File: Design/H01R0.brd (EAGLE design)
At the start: 34.6 x 30 mm, 27 parts, among them P1 HEXABIT_17.32, Q1 MMBT3904LT1, Q2 MMBT3904LT1, Q3 MMBT3904LT1, U1 STM32G0B1CEU6NUFQFPN48_STM32_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, X1 XTALL_CSTCE8M00G52

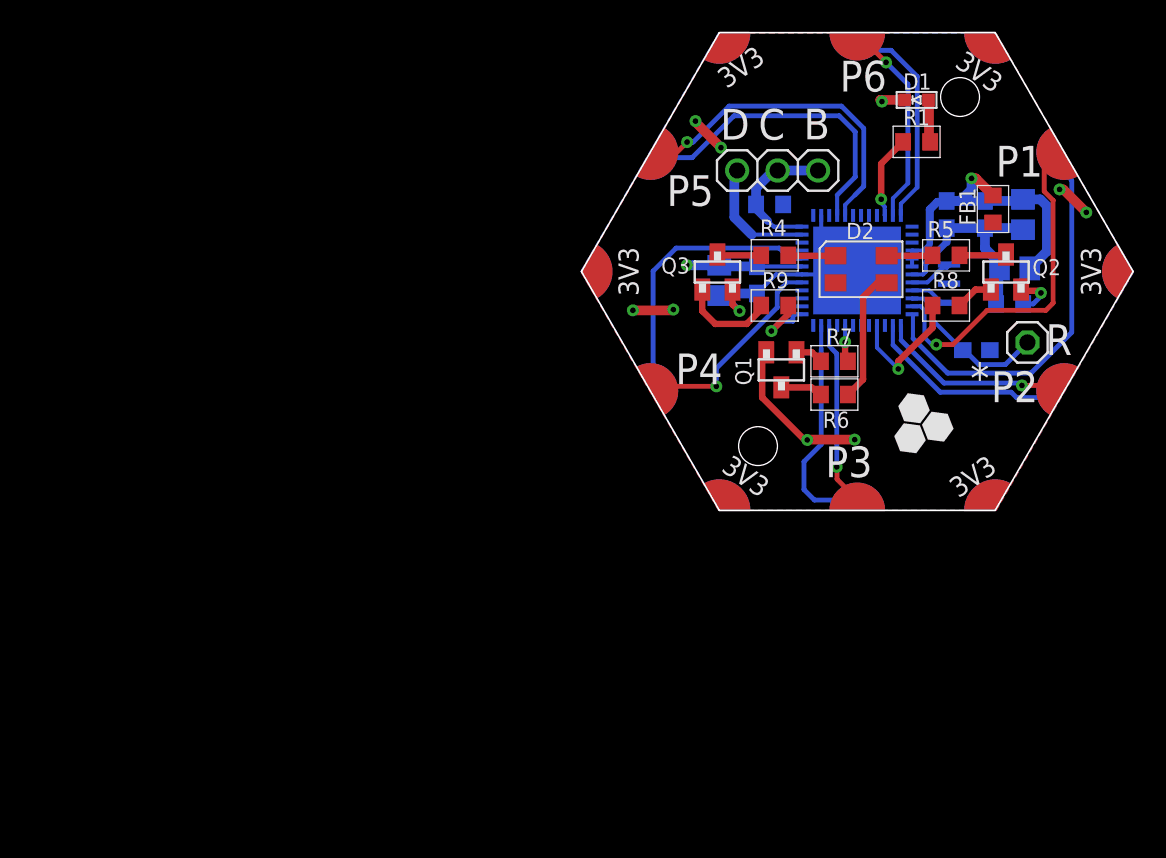
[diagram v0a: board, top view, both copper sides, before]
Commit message: -Improving the Layout Design
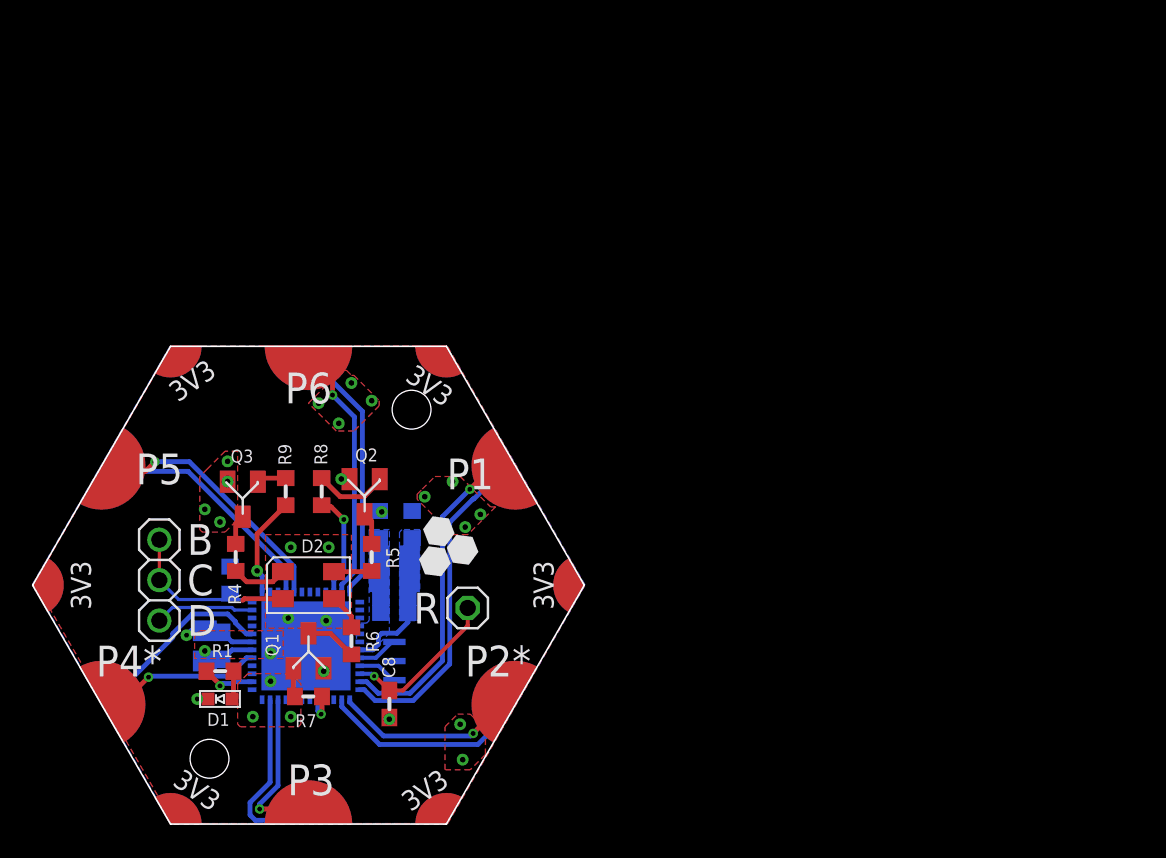
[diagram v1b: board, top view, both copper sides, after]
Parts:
- D1: value VLMS1300-GS08 -> RED
- FB1: device HEXABITZ_RCLS:FB-TDK_MMZ1608Y300B -> HEXABITZ_RCLS:FB-0603
- U1: value STM32G0B1CEU6NUFQFPN48_STM32_STM -> STM32G0B1CEU6N; device HEXABITZ_ICs:UFQFPN48_STM32_STM -> HEXABITZ_ICs:HEXABITZ_ICS_QFN_B1CEU6_STM-L
- moved D1 57.7 mm to (-5.56, 7.78)
- moved R1 54.9 mm to (-5.56, 9.53)
- moved JP2 46.6 mm to (-9.37, 15.2), turned to 270 degrees
- moved C2 45.7 mm to (5.40, 15.2), turned to 180 degrees
- moved C6 44.2 mm to (5.40, 14.1), turned to 180 degrees
- moved FB1 43.3 mm to (4.45, 18.7), flipped to the bottom, turned to 90 degrees
- moved C8 43.0 mm to (5.08, 7.46), flipped to the top, turned to 270 degrees
- moved C7 43.0 mm to (5.40, 16.7), turned to 180 degrees
- moved C5 42.8 mm to (5.40, 13.2), turned to 180 degrees
- moved Q2 42.7 mm to (3.53, 20.5), turned to 180 degrees
- moved X1 42.1 mm to (5.40, 10.2)
- moved U1 41.9 mm to (-0.16, 11.1)
- moved R3 41.3 mm to (-4.92, 15.2), turned to 270 degrees
- moved R8 40.9 mm to (0.83, 20.8), turned to 90 degrees
- moved R5 40.8 mm to (3.97, 16.7), turned to 90 degrees
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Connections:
- net BLED: now also U1.17; no longer U1.20
- net GLED: now also U1.46; no longer U1.16
- net GND: no longer U1.1, U1.2, U1.37, U1.38
- net N$7: now also U1.26; no longer U1.46
- net RLED: now also U1.37; no longer U1.25
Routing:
- net GND: track 33.1 -> 4.73 mm, vias 11 -> 27
- net VDDA: track 21.0 -> 0.00 mm, vias 1 -> 0
- net VSSA: track 14.3 -> 4.60 mm
- net USART4_RX: track 29.7 -> 20.6 mm
- net N$8: track 8.36 -> 2.25 mm
- net USART1_RX: track 17.7 -> 11.8 mm
- net USART3_RX: track 17.1 -> 11.8 mm
- net USART5_TX: track 21.4 -> 16.1 mm
- net USART5_RX: track 19.5 -> 15.0 mm
- net N$15: track 6.01 -> 1.84 mm
- net USART6_TX: track 12.9 -> 16.3 mm
- net USART1_TX: track 12.9 -> 9.97 mm
- net USART6_RX: track 13.8 -> 16.5 mm
- net N$14: track 2.38 -> 4.66 mm
- net N$7: track 5.35 -> 3.40 mm
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- added copper zone on layer 1, net GND
- added copper zone on layer 16, net VDDA
- added copper zone on layer 16, net VSSA
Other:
- board text added: "P2*"
- board text added: "P4*"
- board text removed: "*"
- board text removed: "P2"
- board text removed: "P4"
